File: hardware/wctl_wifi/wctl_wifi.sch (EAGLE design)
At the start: 9 parts, among them U1 Value, U2 ESP32-WROOM-32D

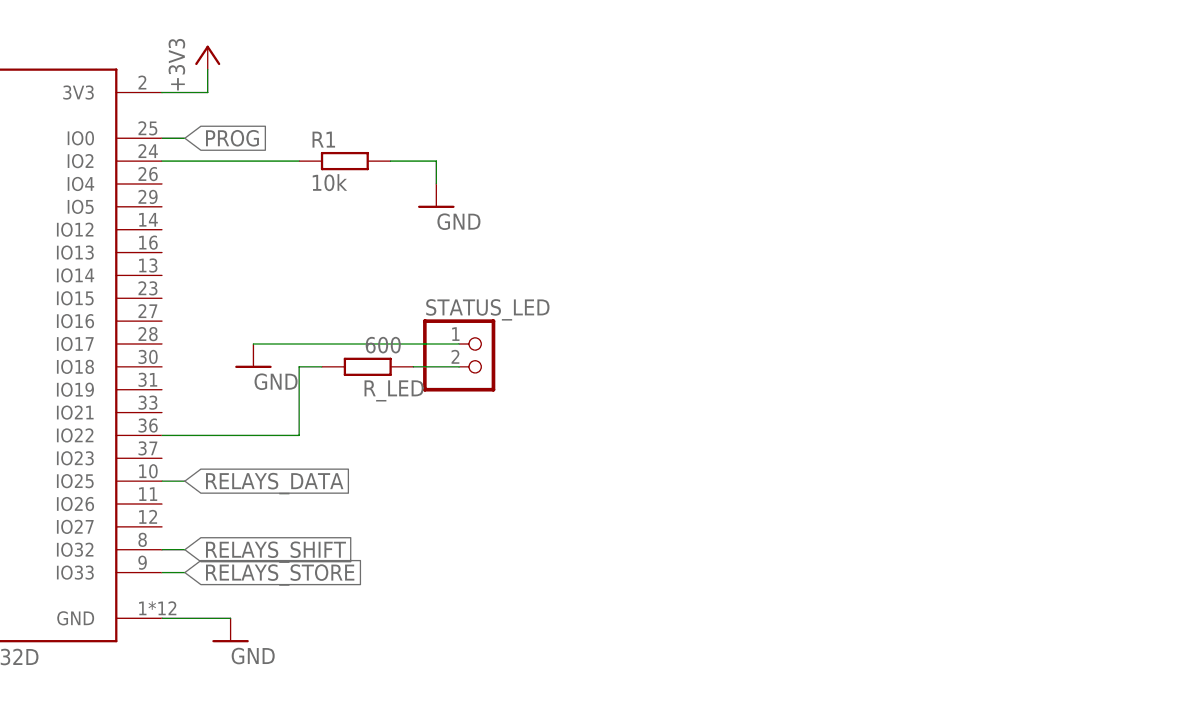
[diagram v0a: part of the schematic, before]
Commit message: hardware: updated wifi board
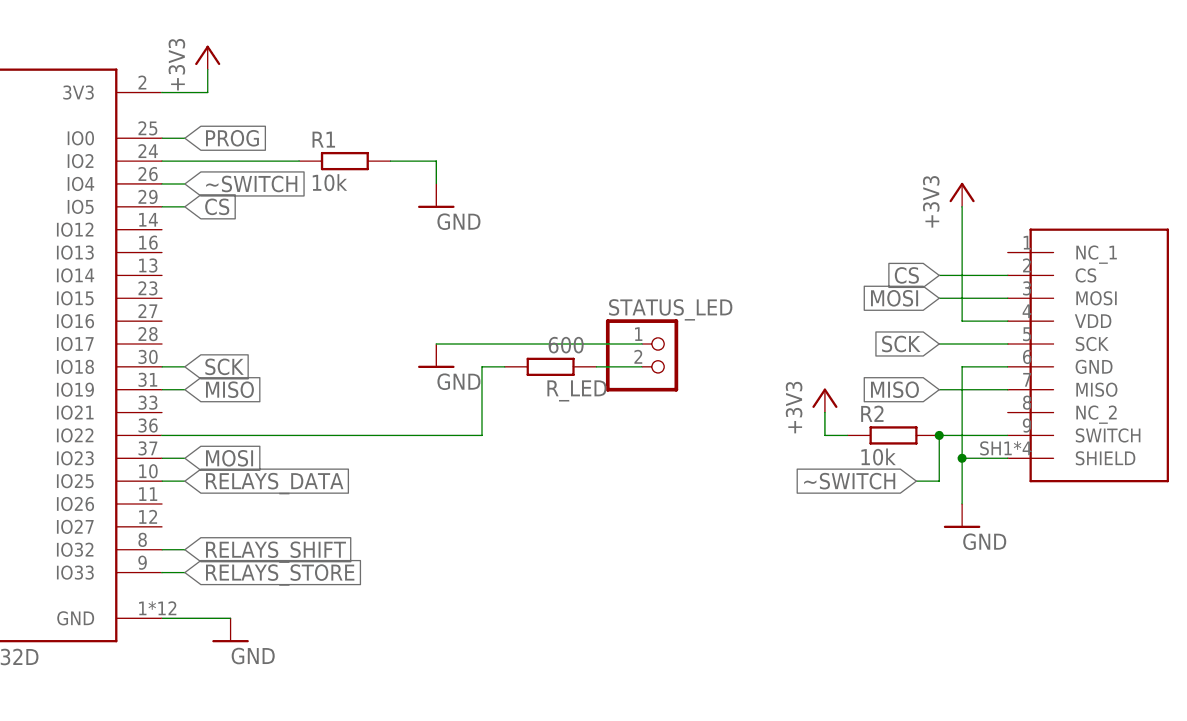
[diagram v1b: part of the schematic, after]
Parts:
- added R2: 10k, rcl:R-EU_R0603
- added U$1: SD_SLOT, sd_slot:SD_SLOT
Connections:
- new net CS: U$1.CS, U2.IO5
- new net MISO: U$1.MISO, U2.IO19
- new net MOSI: U$1.MOSI, U2.IO23
- new net SCK: U$1.SCK, U2.IO18
- new net ~SWITCH: R2.2, U$1.SWITCH, U2.IO4
- net +3V3: now also R2.1, U$1.VDD
- net GND: now also U$1.GND, U$1.SHIELD
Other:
- moved on the sheet: R_LED, STATUS_LED
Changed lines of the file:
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@@
 <part name="C1" library="rcl" library_urn="urn:adsk.eagle:library:334" deviceset="C-EU" device="C0603" package3d_urn="urn:adsk.eagle:package:23616/2"/>
 <part name="+3V2" library="supply1" library_urn="urn:adsk.eagle:library:371" deviceset="+3V3" device=""/>
+<part name="U$1" library="sd_slot" deviceset="SD_SLOT" device=""/>
+<part name="GND8" library="supply1" library_urn="urn:adsk.eagle:library:371" deviceset="GND" device=""/>
+<part name="+3V3" library="supply1" library_urn="urn:adsk.eagle:library:371" deviceset="+3V3" device=""/>
+<part name="R2" library="rcl" library_urn="urn:adsk.eagle:library:334" deviceset="R-EU_" device="R0603" package3d_urn="urn:adsk.eagle:package:23555/3" value="10k"/>
+<part name="+3V5" library="supply1" library_urn="urn:adsk.eagle:library:371" deviceset="+3V3" device=""/>
 </parts>
 <sheets>
@@
 <attribute name="VALUE" x="-12.7" y="-10.16" size="1.778" layer="96"/>
 </instance>
-<instance part="R_LED" gate="G$1" x="83.82" y="48.26" smashed="yes" rot="R180" grouprefs="MICROCONTROLLER">
-<attribute name="NAME" x="90.17" y="46.7614" size="1.778" layer="95" rot="R180"/>
-<attribute name="VALUE" x="87.63" y="51.562" size="1.778" layer="96" rot="R180"/>
-</instance>
-<instance part="GND2" gate="1" x="71.12" y="48.26" smashed="yes" grouprefs="MICROCONTROLLER">
-<attribute name="VALUE" x="71.12" y="45.72" size="1.778" layer="96"/>
+<instance part="R_LED" gate="G$1" x="104.14" y="48.26" smashed="yes" rot="R180" grouprefs="MICROCONTROLLER">
+<attribute name="NAME" x="110.49" y="46.7614" size="1.778" layer="95" rot="R180"/>
+<attribute name="VALUE" x="107.95" y="51.562" size="1.778" layer="96" rot="R180"/>
+</instance>
+<instance part="GND2" gate="1" x="91.44" y="48.26" smashed="yes" grouprefs="MICROCONTROLLER">
+<attribute name="VALUE" x="91.44" y="45.72" size="1.778" layer="96"/>
 </instance>
 <instance part="RELAYS" gate="A" x="10.16" y="-10.16" smashed="yes" rot="R180" grouprefs="RELAYS_INTERFACE">
@@
 <attribute name="VALUE" x="17.78" y="-7.62" size="1.778" layer="96" rot="R90"/>
 </instance>
-<instance part="STATUS_LED" gate="G$1" x="96.52" y="48.26" smashed="yes" grouprefs="MICROCONTROLLER">
-<attribute name="NAME" x="90.17" y="53.975" size="1.778" layer="95"/>
-<attribute name="VALUE" x="90.17" y="43.18" size="1.778" layer="96"/>
+<instance part="STATUS_LED" gate="G$1" x="116.84" y="48.26" smashed="yes" grouprefs="MICROCONTROLLER">
+<attribute name="NAME" x="110.49" y="53.975" size="1.778" layer="95"/>
+<attribute name="VALUE" x="110.49" y="43.18" size="1.778" layer="96"/>
 </instance>
 <instance part="U2" gate="G$1" x="40.64" y="50.8" smashed="yes" grouprefs="MICROCONTROLLER">
@@
 <instance part="+3V2" gate="G$1" x="17.78" y="88.9" smashed="yes">
 <attribute name="VALUE" x="15.24" y="83.82" size="1.778" layer="96" rot="R90"/>
+</instance>
+<instance part="U$1" gate="G$1" x="170.18" y="40.64" smashed="yes" grouprefs="MICROCONTROLLER"/>
+<instance part="GND8" gate="1" x="149.86" y="30.48" smashed="yes" grouprefs="MICROCONTROLLER">
+<attribute name="VALUE" x="149.86" y="27.94" size="1.778" layer="96"/>
+</instance>
+<instance part="+3V3" gate="G$1" x="149.86" y="68.58" smashed="yes" grouprefs="MICROCONTROLLER">
+<attribute name="VALUE" x="147.32" y="63.5" size="1.778" layer="96" rot="R90"/>
+</instance>
+<instance part="R2" gate="G$1" x="142.24" y="40.64" smashed="yes" grouprefs="MICROCONTROLLER">
+<attribute name="NAME" x="138.43" y="42.1386" size="1.778" layer="95"/>
+<attribute name="VALUE" x="138.43" y="37.338" size="1.778" layer="96"/>
+</instance>
+<instance part="+3V5" gate="G$1" x="134.62" y="45.72" smashed="yes" grouprefs="MICROCONTROLLER">
+<attribute name="VALUE" x="132.08" y="40.64" size="1.778" layer="96" rot="R90"/>
 </instance>
 </instances>
@@
 <pinref part="STATUS_LED" gate="G$1" pin="1"/>
 <pinref part="GND2" gate="1" pin="GND"/>
-<wire x1="93.98" y1="50.8" x2="71.12" y2="50.8" width="0.1524" layer="91" grouprefs="MICROCONTROLLER"/>
+<wire x1="114.3" y1="50.8" x2="91.44" y2="50.8" width="0.1524" layer="91" grouprefs="MICROCONTROLLER"/>
 </segment>
 <segment>
@@
 <pinref part="GND6" gate="1" pin="GND"/>
 </segment>
+<segment>
+<pinref part="U$1" gate="G$1" pin="SHIELD"/>
+<wire x1="154.94" y1="38.1" x2="149.86" y2="38.1" width="0.1524" layer="91" grouprefs="MICROCONTROLLER"/>
+<pinref part="GND8" gate="1" pin="GND"/>
+<wire x1="149.86" y1="38.1" x2="149.86" y2="33.02" width="0.1524" layer="91" grouprefs="MICROCONTROLLER"/>
+<pinref part="U$1" gate="G$1" pin="GND"/>
+<wire x1="154.94" y1="48.26" x2="149.86" y2="48.26" width="0.1524" layer="91" grouprefs="MICROCONTROLLER"/>
+<wire x1="149.86" y1="48.26" x2="149.86" y2="38.1" width="0.1524" layer="91" grouprefs="MICROCONTROLLER"/>
+<junction x="149.86" y="38.1" grouprefs="MICROCONTROLLER"/>
+</segment>
 </net>
 <net name="+5V" class="0">
@@
 <pinref part="C1" gate="G$1" pin="1"/>
 <wire x1="17.78" y1="86.36" x2="17.78" y2="83.82" width="0.1524" layer="91"/>
+</segment>
+<segment>
+<pinref part="+3V3" gate="G$1" pin="+3V3"/>
+<pinref part="U$1" gate="G$1" pin="VDD"/>
+<wire x1="149.86" y1="66.04" x2="149.86" y2="53.34" width="0.1524" layer="91" grouprefs="MICROCONTROLLER"/>
+<wire x1="149.86" y1="53.34" x2="154.94" y2="53.34" width="0.1524" layer="91" grouprefs="MICROCONTROLLER"/>
+</segment>
+<segment>
+<pinref part="+3V5" gate="G$1" pin="+3V3"/>
+<pinref part="R2" gate="G$1" pin="1"/>
+<wire x1="134.62" y1="43.18" x2="134.62" y2="40.64" width="0.1524" layer="91" grouprefs="MICROCONTROLLER"/>
+<wire x1="134.62" y1="40.64" x2="137.16" y2="40.64" width="0.1524" layer="91" grouprefs="MICROCONTROLLER"/>
 </segment>
 </net>
@@
 <pinref part="R_LED" gate="G$1" pin="1"/>
 <pinref part="STATUS_LED" gate="G$1" pin="2"/>
-<wire x1="88.9" y1="48.26" x2="93.98" y2="48.26" width="0.1524" layer="91" grouprefs="MICROCONTROLLER"/>
+<wire x1="109.22" y1="48.26" x2="114.3" y2="48.26" width="0.1524" layer="91" grouprefs="MICROCONTROLLER"/>
 </segment>
 </net>
@@
 <segment>
 <pinref part="R_LED" gate="G$1" pin="2"/>
-<wire x1="76.2" y1="48.26" x2="78.74" y2="48.26" width="0.1524" layer="91" grouprefs="MICROCONTROLLER"/>
+<wire x1="96.52" y1="48.26" x2="99.06" y2="48.26" width="0.1524" layer="91" grouprefs="MICROCONTROLLER"/>
 <pinref part="U2" gate="G$1" pin="IO22"/>
-<wire x1="60.96" y1="40.64" x2="76.2" y2="40.64" width="0.1524" layer="91" grouprefs="MICROCONTROLLER"/>
-<wire x1="76.2" y1="40.64" x2="76.2" y2="48.26" width="0.1524" layer="91" grouprefs="MICROCONTROLLER"/>
+<wire x1="60.96" y1="40.64" x2="96.52" y2="40.64" width="0.1524" layer="91" grouprefs="MICROCONTROLLER"/>
+<wire x1="96.52" y1="40.64" x2="96.52" y2="48.26" width="0.1524" layer="91" grouprefs="MICROCONTROLLER"/>
 </segment>
 </net>
@@
 </segment>
 </net>
+<net name="~SWITCH" class="0">
+<segment>
+<pinref part="U$1" gate="G$1" pin="SWITCH"/>
+<wire x1="154.94" y1="40.64" x2="147.32" y2="40.64" width="0.1524" layer="91" grouprefs="MICROCONTROLLER"/>
+<pinref part="R2" gate="G$1" pin="2"/>
+<wire x1="147.32" y1="40.64" x2="147.32" y2="35.56" width="0.1524" layer="91" grouprefs="MICROCONTROLLER"/>
+<junction x="147.32" y="40.64" grouprefs="MICROCONTROLLER"/>
+<wire x1="147.32" y1="35.56" x2="144.78" y2="35.56" width="0.1524" layer="91" grouprefs="MICROCONTROLLER"/>
+<label x="144.78" y="35.56" size="1.778" layer="95" rot="R180" xref="yes" grouprefs="MICROCONTROLLER"/>
+</segment>
+<segment>
+<pinref part="U2" gate="G$1" pin="IO4"/>
+<wire x1="60.96" y1="68.58" x2="63.5" y2="68.58" width="0.1524" layer="91" grouprefs="MICROCONTROLLER"/>
+<label x="63.5" y="68.58" size="1.778" layer="95" xref="yes" grouprefs="MICROCONTROLLER"/>
+</segment>
+</net>
+<net name="MISO" class="0">
+<segment>
+<pinref part="U$1" gate="G$1" pin="MISO"/>
+<wire x1="154.94" y1="45.72" x2="147.32" y2="45.72" width="0.1524" layer="91" grouprefs="MICROCONTROLLER"/>
+<label x="147.32" y="45.72" size="1.778" layer="95" rot="R180" xref="yes" grouprefs="MICROCONTROLLER"/>
+</segment>
+<segment>
+<pinref part="U2" gate="G$1" pin="IO19"/>
+<wire x1="60.96" y1="45.72" x2="63.5" y2="45.72" width="0.1524" layer="91" grouprefs="MICROCONTROLLER"/>
+<label x="63.5" y="45.72" size="1.778" layer="95" xref="yes" grouprefs="MICROCONTROLLER"/>
+</segment>
+</net>
+<net name="SCK" class="0">
+<segment>
+<pinref part="U$1" gate="G$1" pin="SCK"/>
+<wire x1="154.94" y1="50.8" x2="147.32" y2="50.8" width="0.1524" layer="91" grouprefs="MICROCONTROLLER"/>
+<label x="147.32" y="50.8" size="1.778" layer="95" rot="R180" xref="yes" grouprefs="MICROCONTROLLER"/>
+</segment>
+<segment>
+<pinref part="U2" gate="G$1" pin="IO18"/>
+<wire x1="60.96" y1="48.26" x2="63.5" y2="48.26" width="0.1524" layer="91" grouprefs="MICROCONTROLLER"/>
+<label x="63.5" y="48.26" size="1.778" layer="95" xref="yes" grouprefs="MICROCONTROLLER"/>
+</segment>
+</net>
+<net name="MOSI" class="0">
+<segment>
+<pinref part="U$1" gate="G$1" pin="MOSI"/>
+<wire x1="154.94" y1="55.88" x2="147.32" y2="55.88" width="0.1524" layer="91" grouprefs="MICROCONTROLLER"/>
+<label x="147.32" y="55.88" size="1.778" layer="95" rot="R180" xref="yes" grouprefs="MICROCONTROLLER"/>
+</segment>
+<segment>
+<pinref part="U2" gate="G$1" pin="IO23"/>
+<wire x1="60.96" y1="38.1" x2="63.5" y2="38.1" width="0.1524" layer="91" grouprefs="MICROCONTROLLER"/>
+<label x="63.5" y="38.1" size="1.778" layer="95" xref="yes" grouprefs="MICROCONTROLLER"/>
+</segment>
+</net>
+<net name="CS" class="0">
+<segment>
+<pinref part="U$1" gate="G$1" pin="CS"/>
+<wire x1="154.94" y1="58.42" x2="147.32" y2="58.42" width="0.1524" layer="91" grouprefs="MICROCONTROLLER"/>
+<label x="147.32" y="58.42" size="1.778" layer="95" rot="R180" xref="yes" grouprefs="MICROCONTROLLER"/>
+</segment>
+<segment>
+<pinref part="U2" gate="G$1" pin="IO5"/>
+<wire x1="60.96" y1="66.04" x2="63.5" y2="66.04" width="0.1524" layer="91" grouprefs="MICROCONTROLLER"/>
+<label x="63.5" y="66.04" size="1.778" layer="95" xref="yes" grouprefs="MICROCONTROLLER"/>
+</segment>
+</net>
